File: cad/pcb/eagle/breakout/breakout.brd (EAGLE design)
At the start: 38 x 31 mm, 9 parts, among them J1 DF12-32-DS, J2 DF12-32-DS

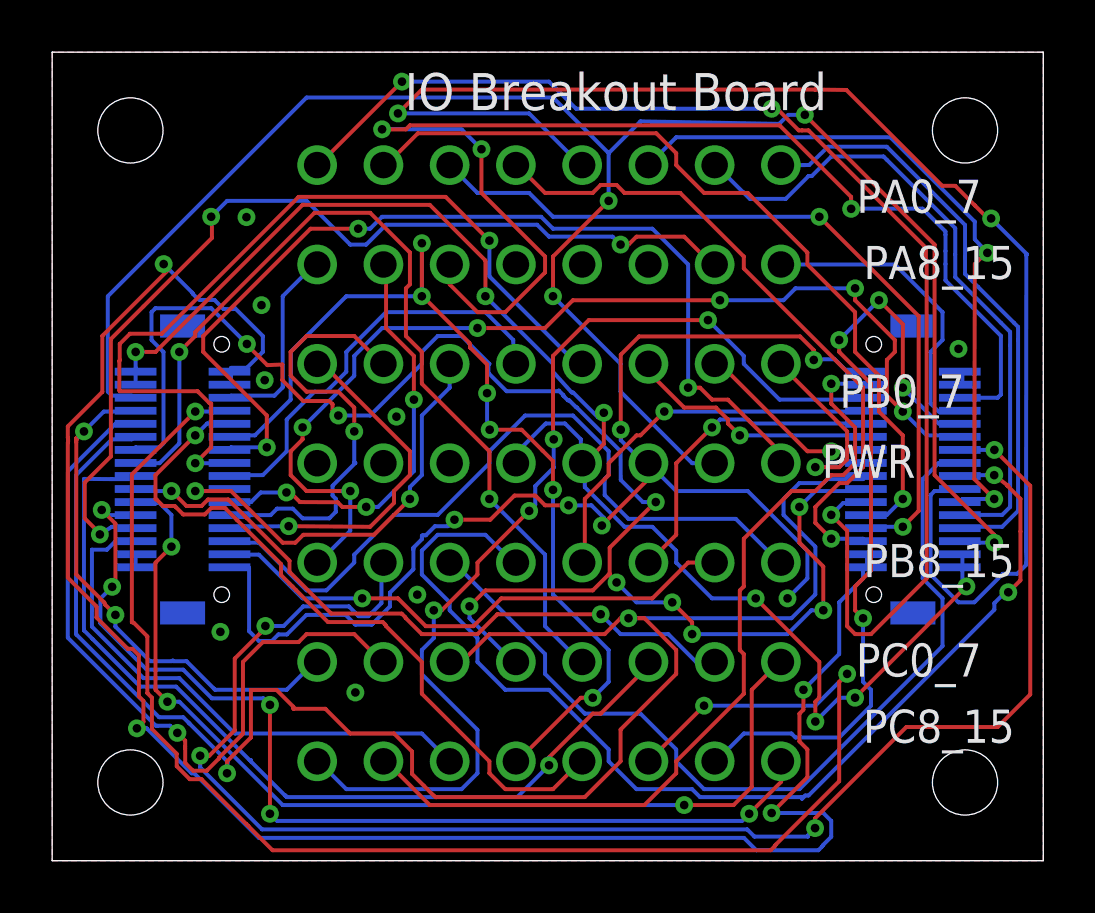
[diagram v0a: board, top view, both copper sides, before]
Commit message: More board tweaks
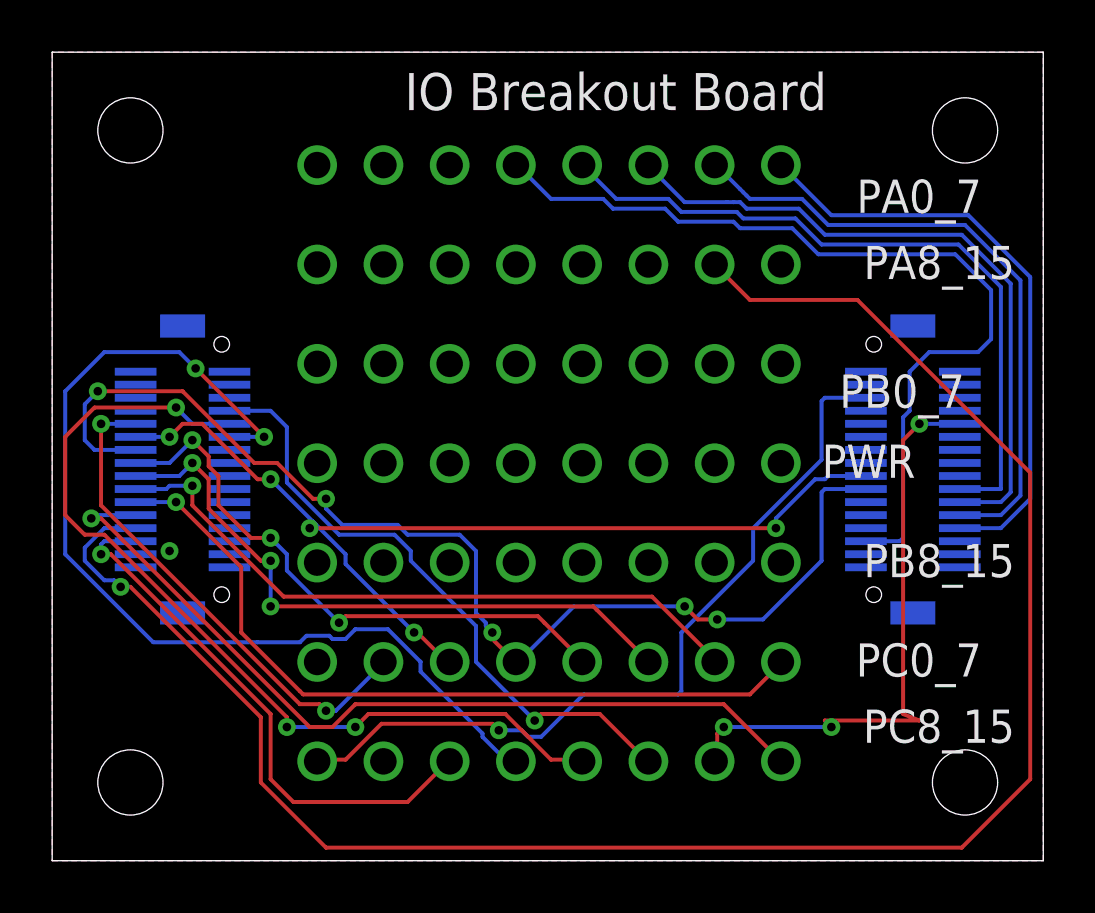
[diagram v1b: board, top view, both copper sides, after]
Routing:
- net PWR_ON: track 72.8 -> 0.00 mm, vias 4 -> 0
- net VCC_3V3: track 72.2 -> 0.00 mm, vias 4 -> 0
- net PB14: track 60.1 -> 0.00 mm, vias 4 -> 0
- net VCC: track 58.5 -> 0.00 mm, vias 7 -> 0
- net PA7: track 50.1 -> 0.00 mm, vias 3 -> 0
- net RESET#: track 49.3 -> 0.00 mm, vias 6 -> 0
- net PA13: track 47.7 -> 0.00 mm, vias 3 -> 0
- net PB12: track 42.3 -> 0.00 mm, vias 2 -> 0
- net PB15: track 40.0 -> 0.00 mm, vias 6 -> 0
- net PD2: track 37.8 -> 0.00 mm, vias 3 -> 0
- net PA9: track 37.6 -> 73.3 mm, vias 3 -> 1
- net PB13: track 33.9 -> 0.00 mm
- net PC10: track 57.8 -> 24.1 mm, vias 3 -> 1
- net PB3: track 32.9 -> 0.00 mm, vias 2 -> 0
- net RSV0: track 32.8 -> 0.07 mm, vias 1 -> 0
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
